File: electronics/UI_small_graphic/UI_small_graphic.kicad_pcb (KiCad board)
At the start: 2 copper layers, 50 x 50 mm, 20 parts, among them J1 Conn_01x06, U1 128x32, U2 128x64, U3 PCF8574, U4 PCA9554

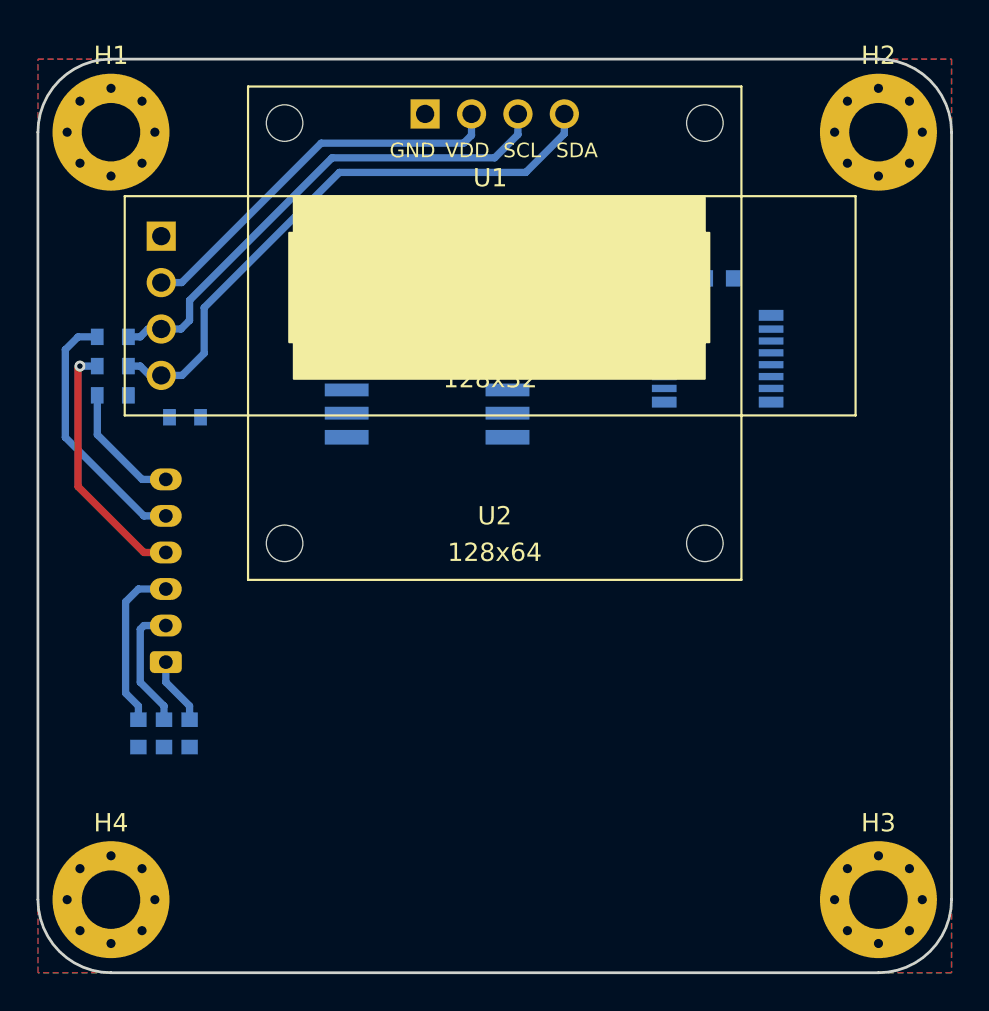
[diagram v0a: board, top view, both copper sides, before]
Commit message: routing
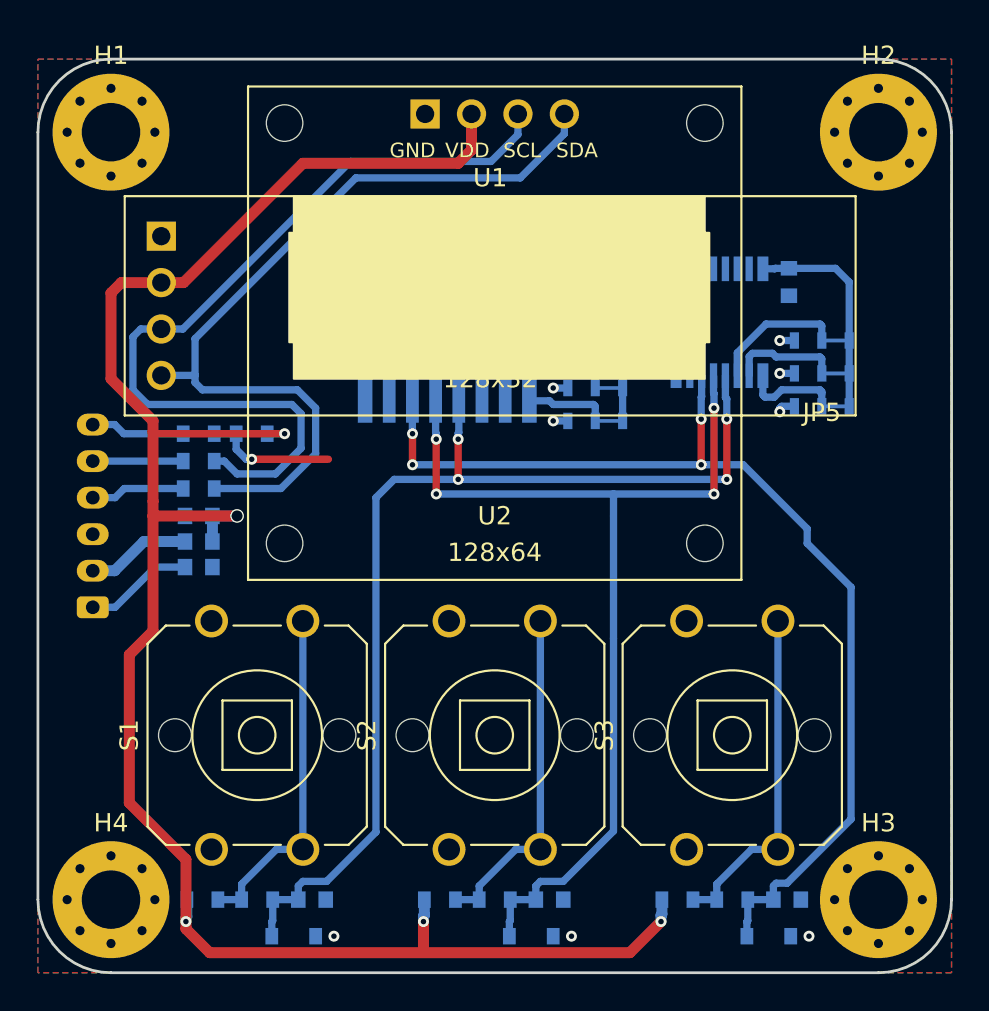
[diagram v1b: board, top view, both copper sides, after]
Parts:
- added C4: 100n, SquantorRcl:C_0603, B.Cu at (165.0, 96.0)
- added C5: 100n, SquantorRcl:C_0603, B.Cu at (178.0, 96.0)
- added C6: 100n, SquantorRcl:C_0603, B.Cu at (191.0, 96.0)
- added D1: SD05, SquantorDiodes:SOD_323_onsemi, B.Cu at (164.0, 98.0)
- added D2: SD05, SquantorDiodes:SOD_323_onsemi, B.Cu at (177.0, 98.0)
- added D3: SD05, SquantorDiodes:SOD_323_onsemi, B.Cu at (190.0, 98.0)
- added JP1: A0, SquantorSpecial:solder_jumper_0603_3way_12conn, B.Cu at (180.5, 69.8)
- added JP2: A1, SquantorSpecial:solder_jumper_0603_3way_12conn, B.Cu at (180.5, 68.0)
- added JP3: A2, SquantorSpecial:solder_jumper_0603_3way_12conn, B.Cu at (180.5, 66.1)
- added JP4: A0, SquantorSpecial:solder_jumper_0603_3way_12conn, B.Cu at (192.9, 69.0)
- added JP5: A1, SquantorSpecial:solder_jumper_0603_3way_12conn, B.Cu at (192.9, 67.2)
- added JP6: A2, SquantorSpecial:solder_jumper_0603_3way_12conn, B.Cu at (192.9, 65.4)
- added R10: 4.7K, SquantorRcl:R_0603_hand, B.Cu at (185.0, 96.0)
- added R5: 100, SquantorRcl:R_0603_hand, B.Cu at (162.0, 96.0)
- added R6: 4.7K, SquantorRcl:R_0603_hand, B.Cu at (159.0, 96.0)
- added R7: 100, SquantorRcl:R_0603_hand, B.Cu at (175.0, 96.0)
- added R8: 100, SquantorRcl:R_0603_hand, B.Cu at (188.0, 96.0)
- added R9: 4.7K, SquantorRcl:R_0603_hand, B.Cu at (172.0, 96.0)
- added S1: BUT0, SquantorSwitches:Omron_B3F-4055, F.Cu at (162.0, 87.0)
- added S2: BUT1, SquantorSwitches:Omron_B3F-4055, F.Cu at (175.0, 87.0)
- added S3: BUT2, SquantorSwitches:Omron_B3F-4055, F.Cu at (188.0, 87.0)
- moved C1 12.3 mm to (158.8, 75.0), turned to 0 degrees
- moved FB1 10.7 mm to (158.8, 76.4), turned to 180 degrees
- moved FB2 9.11 mm to (158.8, 77.8), turned to 180 degrees
- moved C3 8.42 mm to (179.0, 60.7), turned to 270 degrees
- moved R2 8.27 mm to (158.8, 72.0)
- moved R1 8.18 mm to (158.8, 73.5)
- moved N2 7.86 mm to (175.9, 88.3)
- moved N1 5.70 mm to (174.9, 84.3)
- moved R3 5.15 mm to (158.8, 70.5)
- moved J1 5.00 mm to (153.0, 80.0)
- moved C2 3.81 mm to (191.1, 62.2), turned to 270 degrees
- moved R4 3.76 mm to (161.7, 70.5)
- moved U3 2.20 mm to (172.4, 64.3), turned to 90 degrees
- moved U4 2.00 mm to (187.3, 64.4), turned to 90 degrees
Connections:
- net /BUTTON0 renamed /BUTT0
- net /BUTTON1 renamed /BUTT1
- net /BUTTON2 renamed /BUTT2
- net /BUTTON3 renamed /BUTT3
- U3 pad 10: /BUTTON4 -> Net-(U3-Pad10)
- U3 pad 11: /BUTTON4 -> Net-(U3-Pad11)
- U3 pad 9: /BUTTON4 -> Net-(U3-Pad9)
- U4 pad 10: /BUTTON4 -> Net-(U4-Pad10)
- U4 pad 11: /BUTTON4 -> Net-(U4-Pad11)
- U4 pad 9: /BUTTON4 -> Net-(U4-Pad9)
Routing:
- net /3.3V: track 21.5 -> 137.3 mm, vias 0 -> 5
- net /BUTT2: track 0.00 -> 58.3 mm, vias 0 -> 4
- net /BUTT0: track 0.00 -> 57.6 mm, vias 0 -> 4
- net /BUTT1: track 0.00 -> 54.7 mm, vias 0 -> 4
- net /SCL: track 27.7 -> 46.9 mm
- net Net-(R5-Pad1): track 0.00 -> 18.8 mm
- net Net-(R10-Pad2): track 0.00 -> 18.8 mm
- net Net-(R7-Pad1): track 0.00 -> 18.7 mm
- net /SDA: track 32.1 -> 46.2 mm
- net Net-(JP3-Pad2): track 0.00 -> 9.45 mm
- net Net-(J1-Pad5): track 14.1 -> 4.95 mm
- net Net-(J1-Pad4): track 13.9 -> 5.16 mm, vias 1 -> 0
- net Net-(JP2-Pad2): track 0.00 -> 7.66 mm
- net Net-(JP6-Pad2): track 0.00 -> 7.37 mm
- net /!INT: track 0.00 -> 7.33 mm, vias 0 -> 1
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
